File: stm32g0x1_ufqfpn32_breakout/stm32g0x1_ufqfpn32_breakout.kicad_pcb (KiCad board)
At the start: 2 copper layers, 18.5 x 62 mm, 10 parts, among them J1 Conn_01x24, J2 Conn_01x24, J3 Conn_02x07_Odd_Even, SW1 SW_Push, U1 STM32G071CBTx

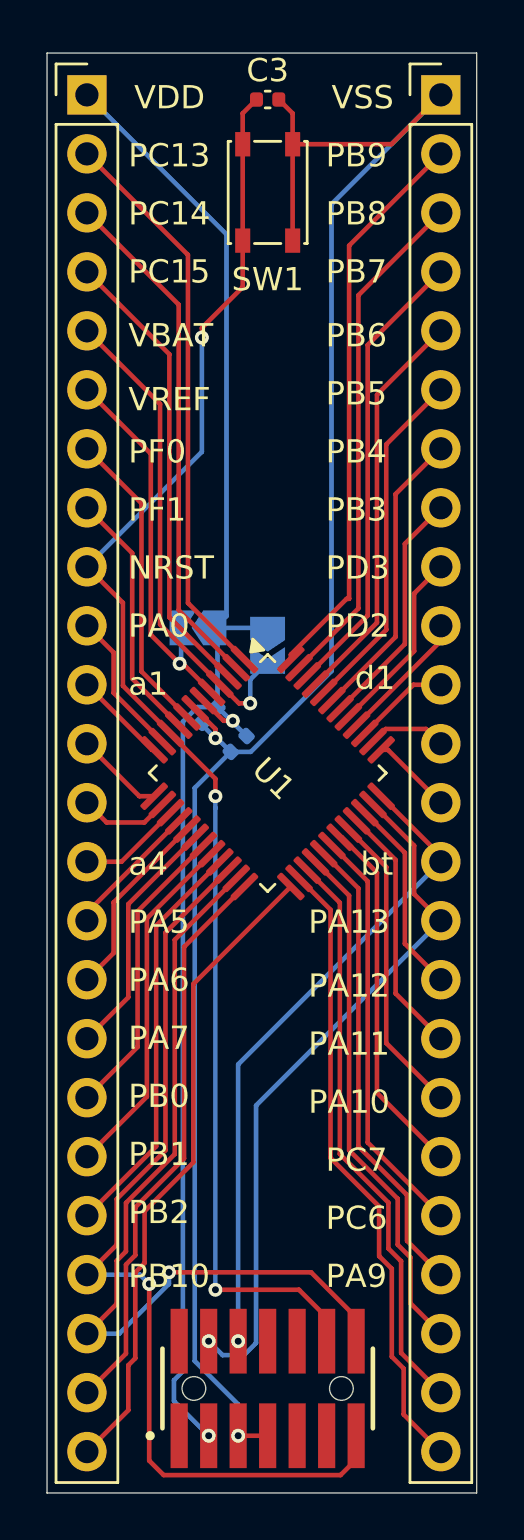
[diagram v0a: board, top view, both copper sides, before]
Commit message: Finalized G0x1 breakouts
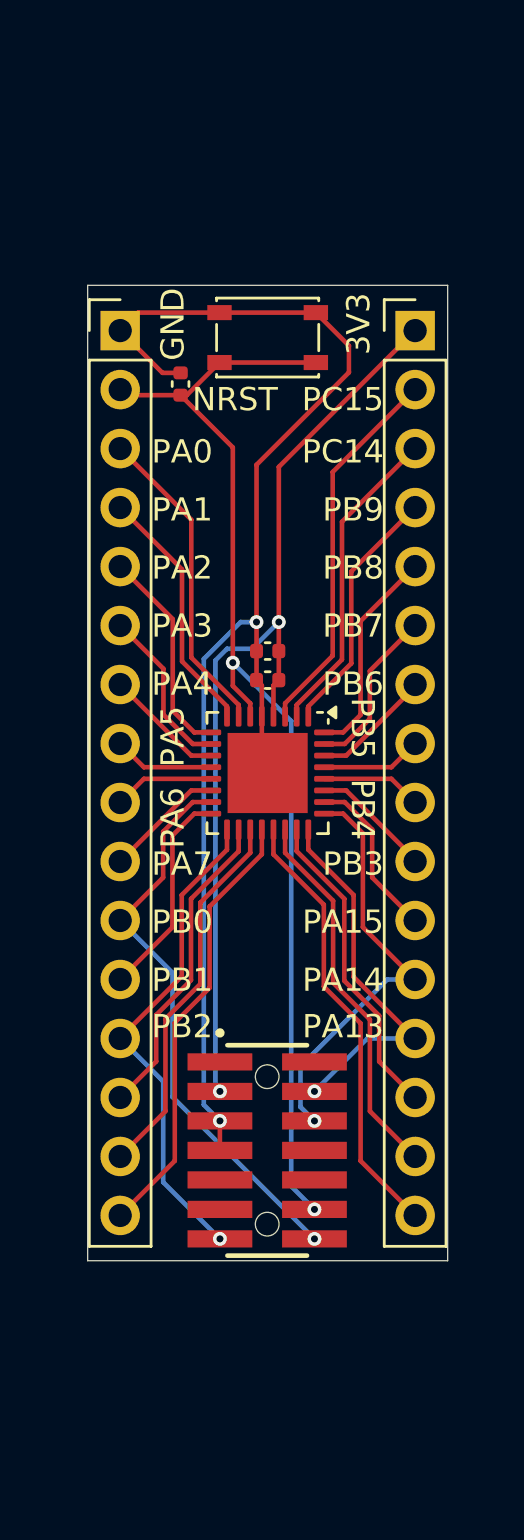
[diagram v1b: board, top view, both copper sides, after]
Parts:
- removed JP1, JP2: SolderJumper_2_Bridged, Jumper:SolderJumper-2_P1.3mm_Open_TrianglePad1.0x1.5mm
- C1, C2: moved to F.Cu
- J1, J2: value Conn_01x24 -> Conn_01x16; footprint Connector_PinHeader_2.54mm:PinHeader_1x24_P2.54mm_Vertical -> Connector_PinHeader_2.54mm:PinHeader_1x16_P2.54mm_Vertical
- U1: value STM32G071CBTx -> STM32G071KBUx; footprint Package_QFP:LQFP-48_7x7mm_P0.5mm -> Package_DFN_QFN:QFN-32-1EP_5x5mm_P0.5mm_EP3.45x3.45mm
- moved C3 12.8 mm to (146.2, 83.2), turned to 90 degrees
- moved J1 10.3 mm to (143.7, 81.0)
- moved J3 10.3 mm to (150.0, 116.2), turned to -90 degrees
- moved J2 10.2 mm to (156.3, 81.0)
- moved SW1 6.25 mm to (150.0, 81.2), turned to 0 degrees
- moved C1 4.19 mm to (150.0, 94.8), turned to 180 degrees
- moved C2 2.92 mm to (150.0, 96.0), turned to 180 degrees
- turned U1 to -90 degrees
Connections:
- J1 pad 1: VDD -> VSS
- J1 pad 10: /PA0 -> /PA7
- J1 pad 11: /PA1 -> /PB0
- J1 pad 12: /PA2 -> /PB1
- J1 pad 13: /PA3 -> /PB2
- J1 pad 14: /PA4 -> /PA8
- J1 pad 15: /PA5 -> /PA9
- J1 pad 16: /PA6 -> /PC6
- J1 pad 2: /PC13 -> /NRST
- J1 pad 3: /PC14 -> /PA0
- J1 pad 4: /PC15 -> /PA1
- J1 pad 5: /VBAT -> /PA2
- J1 pad 6: /VREF -> /PA3
- J1 pad 7: /PF0 -> /PA4
- J1 pad 8: /PF1 -> /PA5
- J1 pad 9: /NRST -> /PA6
- J2 pad 1: VSS -> VDD
- J2 pad 10: /PD2 -> /PB3
- J2 pad 11: /PD1 -> /PA15
- J2 pad 12: /PD0 -> /PA14
- J2 pad 13: /PA15 -> /PA13
- J2 pad 14: /PA14 -> /PA12
- J2 pad 15: /PA13 -> /PA11
- J2 pad 16: /PA12 -> /PA10
- J2 pad 2: /PB9 -> /PC15
- J2 pad 3: /PB8 -> /PC14
- J2 pad 4: /PB7 -> /PB9
- J2 pad 5: /PB6 -> /PB8
- J2 pad 6: /PB5 -> /PB7
- J2 pad 7: /PB4 -> /PB6
- J2 pad 8: /PB3 -> /PB5
- J2 pad 9: /PD3 -> /PB4
- J3 pad 13: /PB10 -> /PB2
- J3 pad 14: /PB11 -> /PB0
- U1 pad 1: /PC13 -> /PB9
- U1 pad 10: /NRST -> /PA3
- U1 pad 11: /PA0 -> /PA4
- U1 pad 12: /PA1 -> /PA5
- U1 pad 13: /PA2 -> /PA6
- U1 pad 14: /PA3 -> /PA7
- U1 pad 15: /PA4 -> /PB0
- U1 pad 16: /PA5 -> /PB1
- U1 pad 17: /PA6 -> /PB2
- U1 pad 18: /PA7 -> /PA8
- U1 pad 19: /PB0 -> /PA9
- U1 pad 20: /PB1 -> /PC6
- U1 pad 21: /PB2 -> /PA10
- U1 pad 22: /PB10 -> /PA11
- U1 pad 23: /PB11 -> /PA12
- U1 pad 24: /PB12 -> /PA13
- U1 pad 25: /PB13 -> /PA14
- U1 pad 26: /PB14 -> /PA15
- U1 pad 27: /PB15 -> /PB3
- U1 pad 28: /PA8 -> /PB4
- U1 pad 29: /PA9 -> /PB5
- U1 pad 30: /PC6 -> /PB6
- U1 pad 31: /PC7 -> /PB7
- U1 pad 32: /PA10 -> /PB8
- U1 pad 33: /PA11 -> VSS
- U1 pad 4: /VBAT -> VDD
- U1 pad 5: /VREF -> VSS
- U1 pad 6: VDD -> /NRST
- U1 pad 7: VSS -> /PA0
- U1 pad 8: /PF0 -> /PA1
- U1 pad 9: /PF1 -> /PA2
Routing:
- net /PB10: track 40.9 -> 0.00 mm, vias 1 -> 0
- net /PB11: track 37.1 -> 0.00 mm, vias 1 -> 0
- net /PB13: track 28.0 -> 0.00 mm
- net /PB14: track 27.2 -> 0.00 mm
- net VDD: track 68.1 -> 41.2 mm
- net /PB15: track 24.9 -> 0.00 mm
- net /PB12: track 24.6 -> 0.00 mm
- net /PC13: track 24.6 -> 0.00 mm
- net VSS: track 81.7 -> 58.7 mm
- net /VBAT: track 21.3 -> 0.00 mm, vias 1 -> 0
- net /VREF: track 16.9 -> 0.00 mm, vias 1 -> 0
- net /PC7: track 15.6 -> 0.00 mm
- net /PA13: track 30.2 -> 16.2 mm
- net /NRST: track 62.9 -> 49.2 mm, vias 3 -> 2
- net /PB9: track 24.5 -> 10.9 mm
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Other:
- board size 18.5 x 62 mm -> 15.5 x 42 mm
- board text added: "3V3"
- board text added: "GND"
- board text added: "PA1"
- board text added: "PA14"
- board text added: "PA15"
- board text added: "PA2"
- board text added: "PA3"
- board text added: "PA4"
- board text removed: "PA10"
- board text removed: "PA11"
- board text removed: "PA12"
- board text removed: "PA9"
- board text removed: "PB10"
- board text removed: "PC13"
- board text removed: "PC6"
- board text removed: "PC7"
- board text removed: "PD2"
- board text removed: "PD3"
- board text removed: "PF0"
- board text removed: "PF1"
- board text removed: "VBAT"
- board text removed: "VDD"
- board text removed: "VREF"
- board text removed: "VSS"
- board text removed: "a1"
- board text removed: "a4"
- board text removed: "bt"
- board text removed: "d1"
